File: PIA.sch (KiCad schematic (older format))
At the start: 0 parts

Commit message: PIA and POKEY
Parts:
- added C68: 100nF, Atari:C_Axial_L5.1mm_D2.5mm_P12.50mm_Horizontal, symbol Device:C
- added C79: 22uF, Capacitor_THT:CP_Radial_D5.0mm_P2.50mm, symbol Device:CP
- added C80, C81, C82, C83, C84, C85, C86, C87, C88, C89, C90, C91, C92: 1nF, Atari:C_Axial_L5.1mm_D2.5mm_P12.50mm_Horizontal, symbol Device:C
- added FB10, FB11: Ferrite_Bead, Atari:L_Axial_L7.0mm_D3.3mm_P12.50mm_Horizontal_Fastron_MICC, symbol Device:Ferrite_Bead
- added L19, L20, L21, L22, L26, L27, L28, L29: 10uH, Atari:L_Axial_L7.0mm_D3.3mm_P12.50mm_Horizontal_Fastron_MICC, symbol Device:L
- added Q4: 2N3906, Package_TO_SOT_THT:TO-92_Wide, symbol Transistor_BJT:2N3906
- added R117, R119: 100, Atari:R_Axial_DIN0207_L3.6mm_D2.2mm_P10.16mm_Horizontal, symbol Device:R
- added R118, R120, R121, R122, R123, R124, R125, R126, R127: 220, Atari:R_Axial_DIN0207_L3.6mm_D2.2mm_P10.16mm_Horizontal, symbol Device:R
- added R206: 3k3, Atari:R_Axial_DIN0207_L3.6mm_D2.2mm_P10.16mm_Horizontal, symbol Device:R
- added R23, R24, R25, R85, R86, R87, R88: 3k, Atari:R_Axial_DIN0207_L3.6mm_D2.2mm_P10.16mm_Horizontal, symbol Device:R
- added R91: 2k7, Atari:R_Axial_DIN0207_L3.6mm_D2.2mm_P10.16mm_Horizontal, symbol Device:R
- added R92, R93, R94: 4k7, Atari:R_Axial_DIN0207_L3.6mm_D2.2mm_P10.16mm_Horizontal, symbol Device:R
- added U23: PIA, Package_DIP:DIP-40_W15.24mm_Socket, symbol Atari:PIA
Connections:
- new net: R118.2, U23.18 (CB1)
- new net: R119.2, R94.1, U23.19 (CB2)
- new net: R120.2, U23.2 (PA0)
- new net: R86.2, U23.22 (CS0), U23.24 (CS1)
- new net: R121.2, U23.3 (PA1)
- new net: R91.2, U23.39 (CA2)
- new net: R122.2, U23.4 (PA2)
- new net: R117.2, R92.2, U23.40 (CA1)
- new net: R123.2, U23.5 (PA3)
- new net: R124.2, U23.6 (PA4)
- new net: R125.2, U23.7 (PA5)
- new net: R126.2, U23.8 (PA6)
- new net: R127.2, U23.9 (PA7)
- new net: C85.1, L29.2, R120.1
- new net: C86.1, L28.2, R121.1
- new net: C87.1, L27.2, R122.1
- new net: C88.1, L26.2, R123.1
- new net: C89.1, L22.2, R124.1
- new net: C90.1, L21.2, R125.1
- new net: C91.1, L20.2, R126.1
- new net: C92.1, L19.2, R127.1
- new net: Q4.2 (B), R91.1
- new net: FB11.2, Q4.3 (C)
- new net +5VA: C68.1, FB10.2, Q4.1 (E), R206.1, R23.1, R24.1, R25.1, R85.1, R86.1, R87.1, R88.1, R92.1, R93.2, R94.2, U23.20 (VCC)
- new net A0: U23.35 (A0)
- new net A1: U23.36 (A1)
- new net BACK0: L28.1
- new net BACK1: L21.1
- new net COMMAND: C84.1, R119.1
- new net D0: U23.33 (D0)
- new net D1: U23.32 (D1)
- new net D2: U23.31 (D2)
- new net D3: U23.30 (D3)
- new net D4: U23.29 (D4)
- new net D5: U23.28 (D5)
- new net D6: U23.27 (D6)
- new net D7: U23.26 (D7)
- new net FWD0: L29.1
- new net FWD1: L22.1
- new net GND: C68.2, C79.2, C80.2, C81.2, C82.2, C83.2, C84.2, C85.2, C86.2, C87.2, C88.2, C89.2, C90.2, C91.2, C92.2, U23.1 (VSS)
- new net INTRUPT: C83.1, R118.1, R93.1
- new net IRQ: U23.37 (~IRQB), U23.38 (~IRQA)
- new net LEFT0: L27.1
- new net LEFT1: L20.1
- new net MTR_CLR: C81.1, FB11.1
- new net O2: U23.25 (O2)
- new net PB0: R88.2, U23.10 (PB0)
- new net PB1: R85.2, U23.11 (PB1)
- new net PB2: R23.2, U23.12 (PB2)
- new net PB3: R25.2, U23.13 (PB3)
- new net PB4: R24.2, U23.14 (PB4)
- new net PB5: R206.2, U23.15 (PB5)
- new net PB7: R87.2, U23.17 (PB7)
- new net PIA: U23.23 (~CS2)
- new net PROCEED: C82.1, R117.1
- new net READY: C79.1, C80.1, FB10.1
- new net RIGHT0: L26.1
- new net RIGHT1: L19.1
- new net RST: U23.34 (~RST)
- new net RW: U23.21 (R/~W)
- no-connect marks 0 -> 1

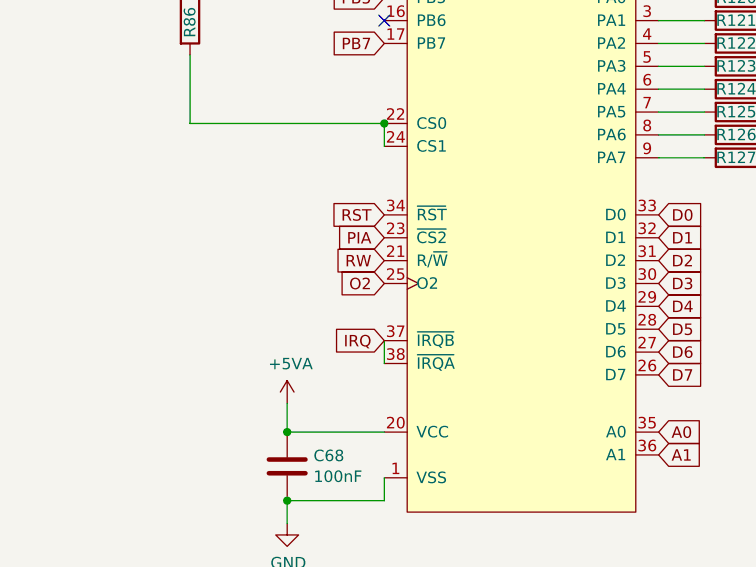
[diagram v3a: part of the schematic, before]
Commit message: Patching
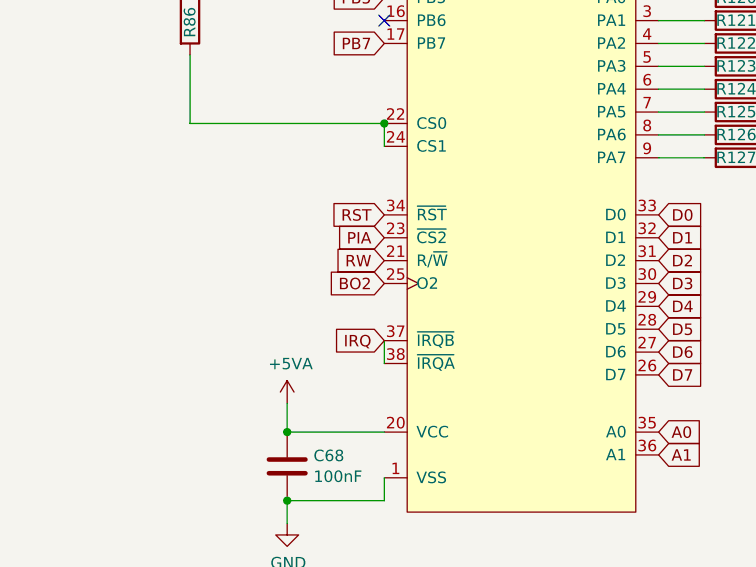
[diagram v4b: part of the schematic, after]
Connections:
- net O2 renamed BO2
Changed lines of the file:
@@
 RW
 Text GLabel 3225 5025 0    50   Input ~ 0
-O2
+BO2
 Text GLabel 3225 4825 0    50   Input ~ 0
 PIA

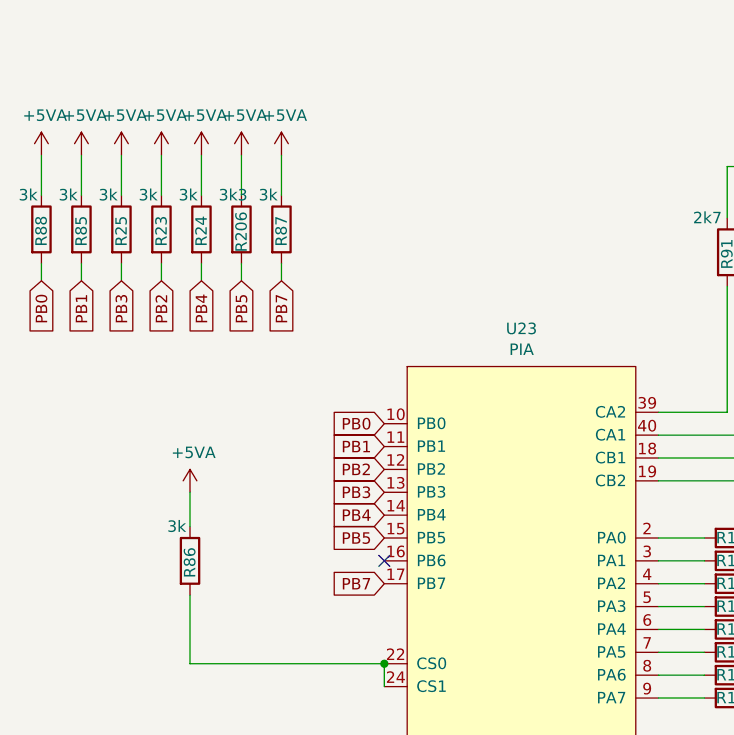
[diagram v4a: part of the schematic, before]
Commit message: Tracking
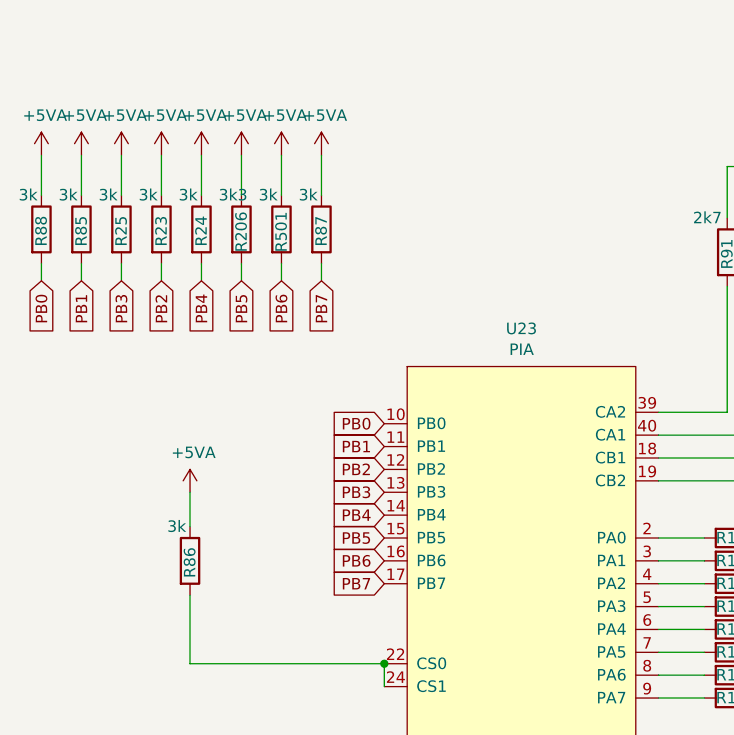
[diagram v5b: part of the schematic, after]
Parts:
- added R501: 3k, Atari:R_Axial_DIN0207_L3.6mm_D2.2mm_P10.16mm_Horizontal, symbol Device:R
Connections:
- net +5VA: now also R501.1
- net PB6: now reaches U23.16 (PB6)
- net PB6: now also R501.2
- no-connect marks 1 -> 0
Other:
- moved on the sheet: R87
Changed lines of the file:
@@
 Text GLabel 3225 3975 0    50   Input ~ 0
 PB7
-NoConn ~ 3225 3875
 Text GLabel 1725 2650 3    50   Input ~ 0
 PB0
@@
 	1    0    0    -1
 $EndComp
-Text GLabel 2775 2650 3    50   Input ~ 0
+Text GLabel 2950 2650 3    50   Input ~ 0
 PB7
 $Comp
 L Device:R R87
 U 1 1 60299733
-P 2775 2425
-F 0 "R87" V 2775 2350 50  0000 L CNN
-F 1 "3k" H 2675 2575 50  0000 L CNN
-F 2 "Atari:R_Axial_DIN0207_L3.6mm_D2.2mm_P10.16mm_Horizontal" V 2705 2425 50  0001 C CNN
-F 3 "~" H 2775 2425 50  0001 C CNN
-	1    2775 2425
+P 2950 2425
+F 0 "R87" V 2950 2350 50  0000 L CNN
+F 1 "3k" H 2850 2575 50  0000 L CNN
+F 2 "Atari:R_Axial_DIN0207_L3.6mm_D2.2mm_P10.16mm_Horizontal" V 2880 2425 50  0001 C CNN
+F 3 "~" H 2950 2425 50  0001 C CNN
+	1    2950 2425
 	1    0    0    -1
 $EndComp
@@
 L power:+5VA #PWR0209
 U 1 1 6029A34C
-P 2775 2100
-F 0 "#PWR0209" H 2775 1950 50  0001 C CNN
-F 1 "+5VA" H 2790 2273 50  0000 C CNN
-F 2 "" H 2775 2100 50  0001 C CNN
-F 3 "" H 2775 2100 50  0001 C CNN
-	1    2775 2100
+P 2950 2100
+F 0 "#PWR0209" H 2950 1950 50  0001 C CNN
+F 1 "+5VA" H 2965 2273 50  0000 C CNN
+F 2 "" H 2950 2100 50  0001 C CNN
+F 3 "" H 2950 2100 50  0001 C CNN
+	1    2950 2100
 	1    0    0    -1
 $EndComp
@@
 	2600 2575 2600 2650
 Wire Wire Line
-	2775 2575 2775 2650
+	2950 2575 2950 2650
 Wire Wire Line
 	1900 2100 1900 2275
@@
 	2600 2100 2600 2275
 Wire Wire Line
-	2775 2100 2775 2275
+	2950 2100 2950 2275
 Text GLabel 3225 4725 0    50   Input ~ 0
 RST
@@
 	8675 5250 8675 5075
 Connection ~ 8675 5075
+Text GLabel 3225 3875 0    50   Input ~ 0
+PB6
+$Comp
+L Device:R R501
+U 1 1 60344EEE
+P 2775 2425
+F 0 "R501" V 2775 2325 50  0000 L CNN
+F 1 "3k" H 2675 2575 50  0000 L CNN
+F 2 "Atari:R_Axial_DIN0207_L3.6mm_D2.2mm_P10.16mm_Horizontal" V 2705 2425 50  0001 C CNN
+F 3 "~" H 2775 2425 50  0001 C CNN
+	1    2775 2425
+	1    0    0    -1
+$EndComp
+Text GLabel 2775 2650 3    50   Input ~ 0
+PB6
+Wire Wire Line
+	2775 2575 2775 2650
+$Comp
+L power:+5VA #PWR0252
+U 1 1 603494C4
+P 2775 2100
+F 0 "#PWR0252" H 2775 1950 50  0001 C CNN
+F 1 "+5VA" H 2790 2273 50  0000 C CNN
+F 2 "" H 2775 2100 50  0001 C CNN
+F 3 "" H 2775 2100 50  0001 C CNN
+	1    2775 2100
+	1    0    0    -1
+$EndComp
+Wire Wire Line
+	2775 2100 2775 2275
 $EndSCHEMATC

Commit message: Gerber and Tracking
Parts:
- C79: footprint Capacitor_THT:CP_Radial_D5.0mm_P2.50mm -> Capacitor_THT:CP_Axial_L11.0mm_D5.0mm_P18.00mm_Horizontal
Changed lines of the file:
@@
 F 0 "C79" H 7218 2446 50  0000 L CNN
 F 1 "22uF" H 7218 2355 50  0000 L CNN
-F 2 "Capacitor_THT:CP_Radial_D5.0mm_P2.50mm" H 7138 2250 50  0001 C CNN
+F 2 "Capacitor_THT:CP_Axial_L11.0mm_D5.0mm_P18.00mm_Horizontal" H 7138 2250 50  0001 C CNN
 F 3 "~" H 7100 2400 50  0001 C CNN
 	1    7100 2400
